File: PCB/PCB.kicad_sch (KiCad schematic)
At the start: 19 parts, among them J1 USB_C_Receptacle_USB2.0_16P, U1 RP2040, U2 USBLC6-2SC6, U3 NCP1117ST33T3G

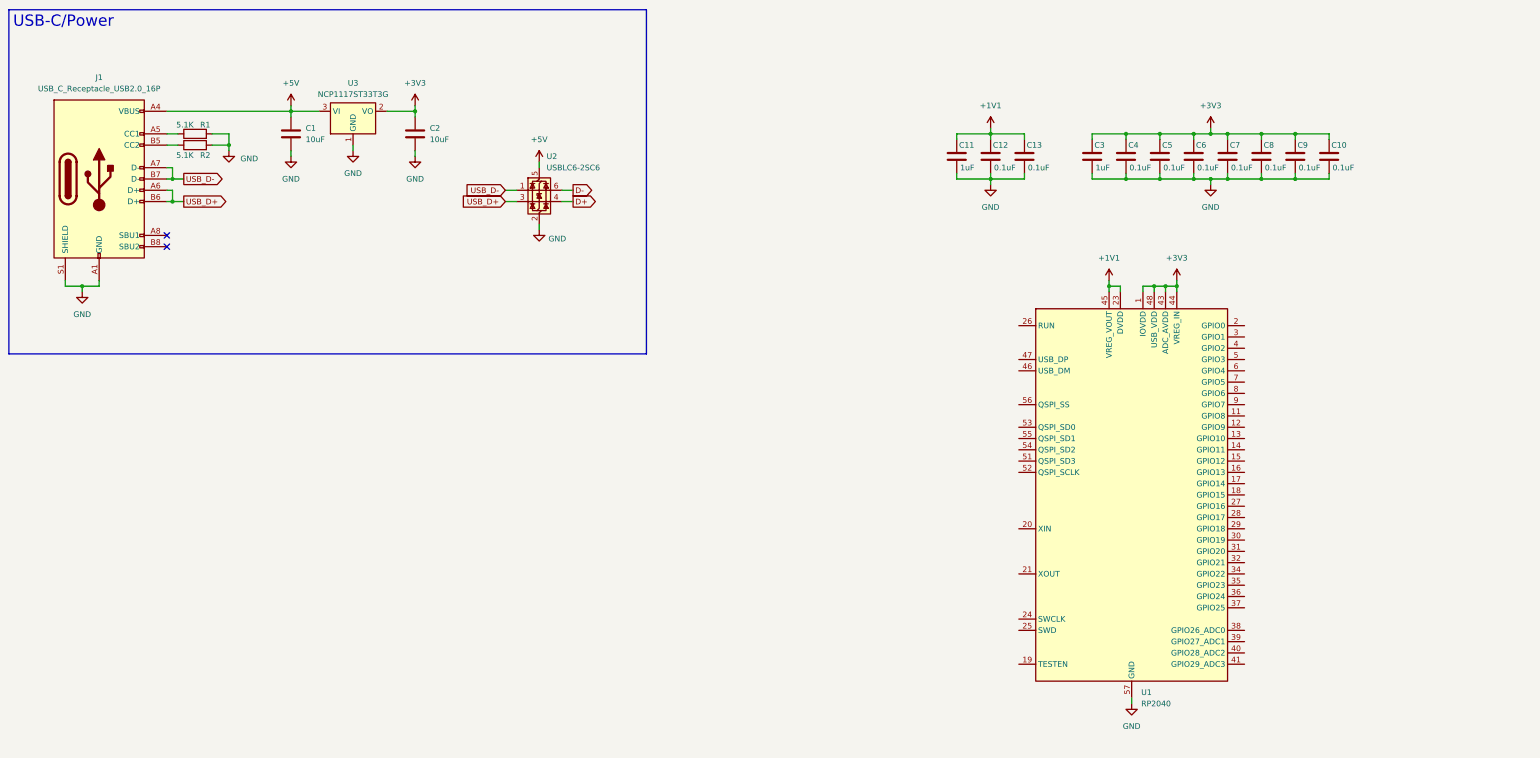
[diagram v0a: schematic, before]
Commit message: crystal and reset
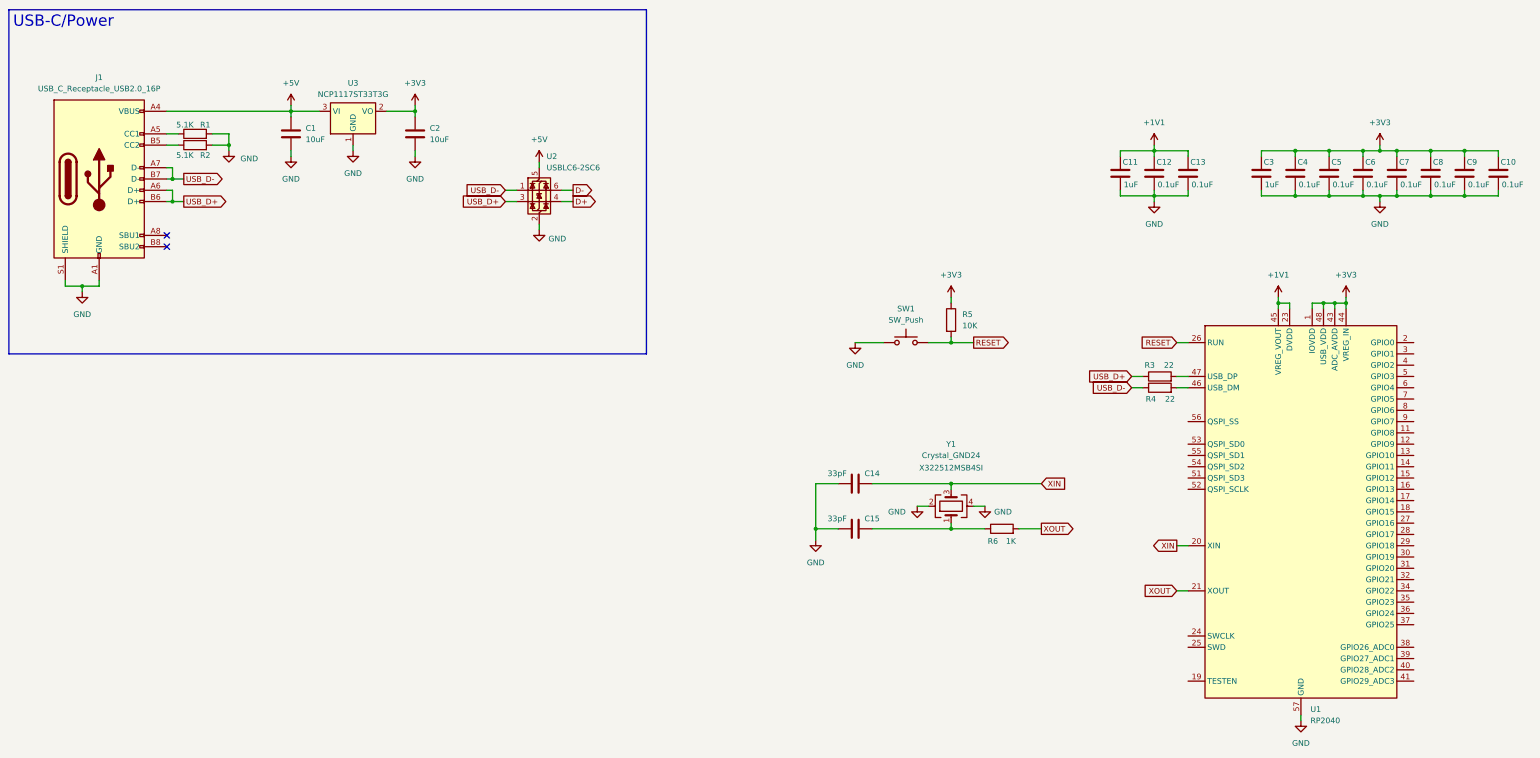
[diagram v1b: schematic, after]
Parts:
- added C14, C15: 33pF, symbol Device:C
- added R3, R4: 22, symbol Device:R
- added R5: 10K, symbol Device:R
- added R6: 1K, symbol Device:R
- added SW1: SW_Push, symbol Switch:SW_Push
- added Y1: Crystal_GND24, symbol Device:Crystal_GND24
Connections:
- net +3V3: now also R5.1
- net GND: now also C14.1, C15.1, SW1.1, Y1.2, Y1.4
- net USB_D+: now also R3.1
- net USB_D-: now also R4.1
- net XIN: now reaches U1.20 (XIN)
- net XIN: now also C14.2, Y1.3
- net XOUT: now reaches U1.21 (XOUT)
- net XOUT: now also R6.2
- net RESET: now reaches U1.26 (RUN)
- net RESET: now also R5.2, SW1.2
- net at U1.46 (USB_DM): now also R4.2
- net at U1.47 (USB_DP): now also R3.2
- new net: C15.2, R6.1, Y1.1
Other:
- moved on the sheet: C10, C11, C12, C13, C3, C4, C5, C6, C7, C8, C9, U1
